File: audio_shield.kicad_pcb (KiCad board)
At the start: 2 copper layers, 11 parts, among them J1 AudioJack2, U1 LM386, U3 OPA340NA

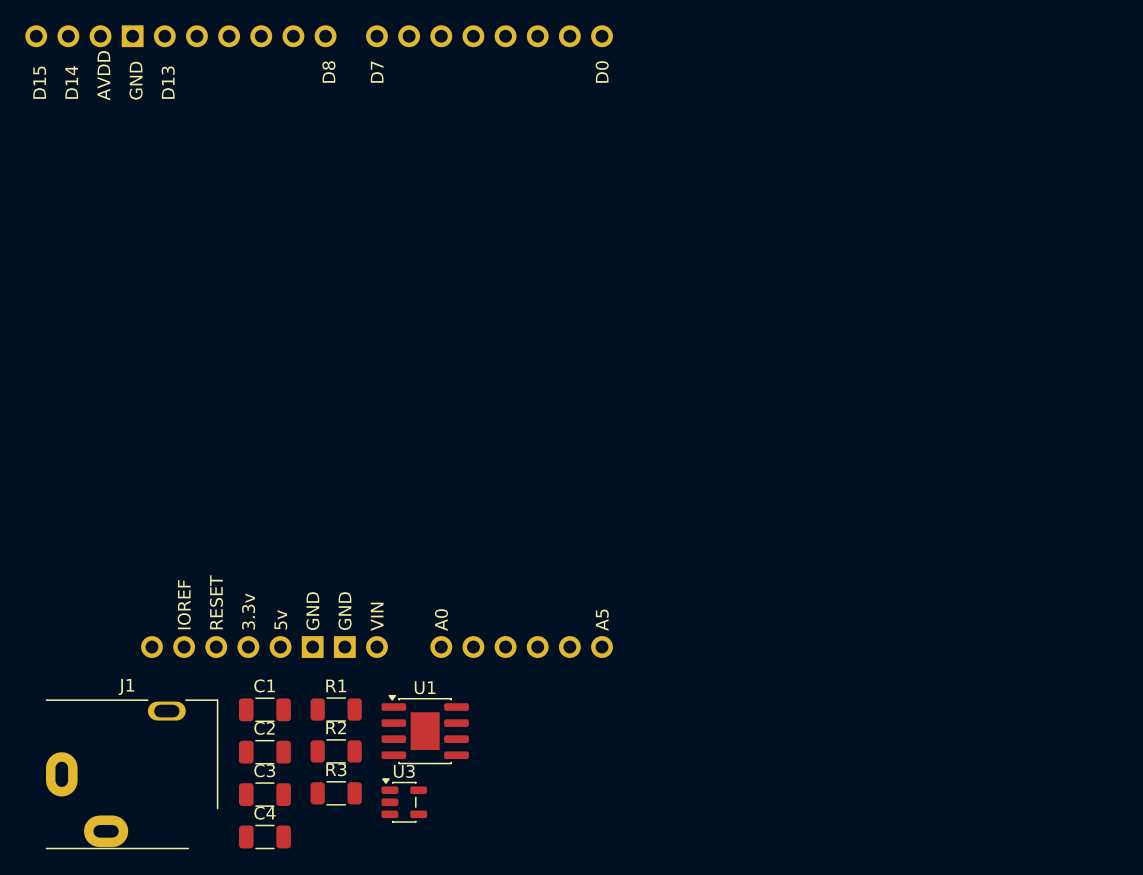
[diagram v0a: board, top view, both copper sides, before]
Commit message: route the board
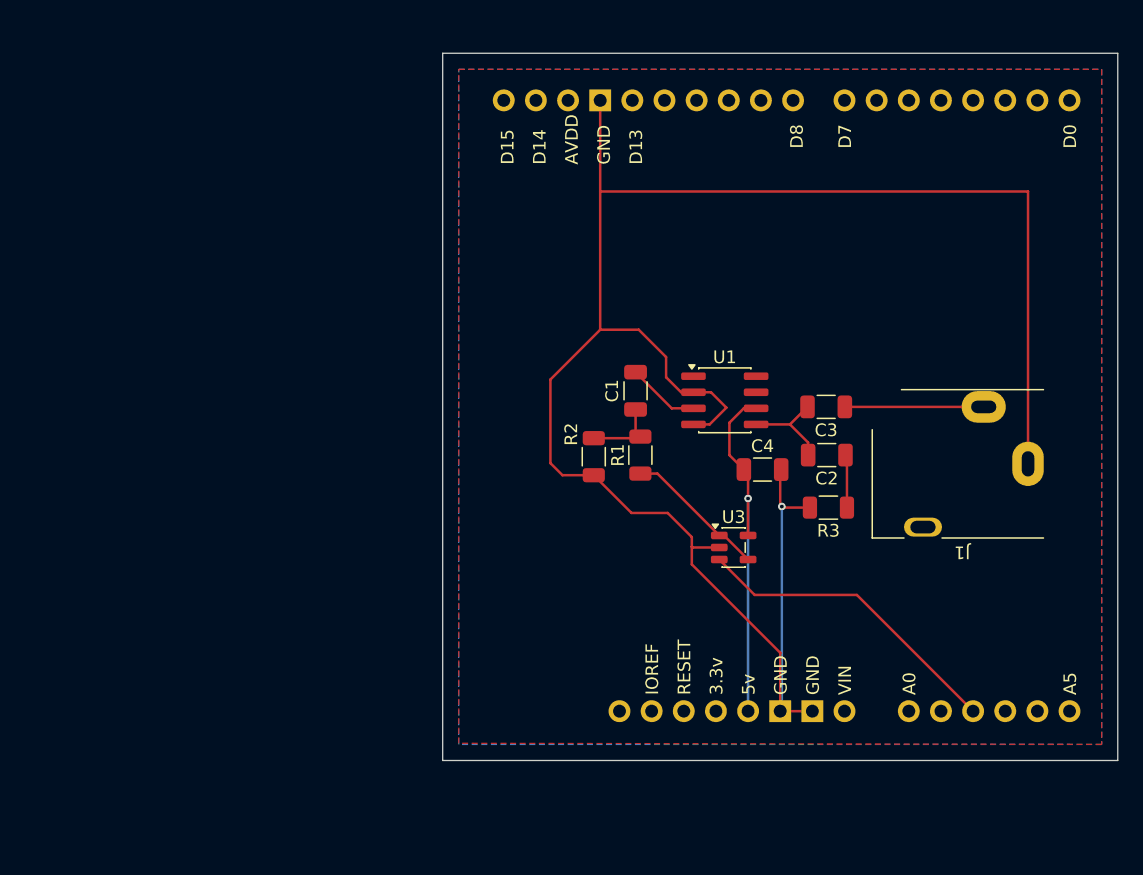
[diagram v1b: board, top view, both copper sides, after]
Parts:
- U1: footprint Package_SO:SOIC-8-1EP_3.9x4.9mm_P1.27mm_EP2.29x3mm -> Package_SO:SOIC-8_3.9x4.9mm_P1.27mm
- moved J1 80.2 mm to (168.2, 93.4), turned to 180 degrees
- moved C3 53.9 mm to (152.2, 88.9), turned to 180 degrees
- moved C2 50.2 mm to (152.3, 92.7), turned to 180 degrees
- moved C4 48.9 mm to (147.2, 93.9)
- moved R3 45.0 mm to (152.4, 96.9), turned to 180 degrees
- moved C1 38.6 mm to (137.2, 87.6), turned to 90 degrees
- moved A1 37.3 mm to (123.2, 115.5)
- moved U1 35.3 mm to (144.2, 88.4)
- moved U3 32.9 mm to (144.9, 100.0)
- moved R1 31.3 mm to (137.5, 92.7), turned to 90 degrees
- moved R2 30.9 mm to (133.9, 92.8), turned to -90 degrees
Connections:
- A1 pad 29: unconnected-(A1-GND-Pad29) -> GND
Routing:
- net GND: track 0.00 -> 158.9 mm, vias 0 -> 1
- net VCC: track 0.00 -> 28.9 mm, vias 0 -> 1
- net /LEFT_DAC: track 0.00 -> 25.0 mm
- net Net-(U3--): track 0.00 -> 11.7 mm
- net /LEFT_SPEAKER: track 0.00 -> 11.0 mm
- net Net-(C2-Pad2): track 0.00 -> 7.65 mm
- net Net-(U1-+): track 0.00 -> 5.76 mm
- net Net-(C1-Pad1): track 0.00 -> 5.50 mm
- net Net-(C2-Pad1): track 0.00 -> 4.20 mm
- added copper zone on B.Cu, net GND
- added copper zone on F.Cu, net GND
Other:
- board outline added: 53.3 x 55.9 mm
